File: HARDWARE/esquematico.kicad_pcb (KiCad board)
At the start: 2 copper layers, 52 parts, among them J1 Screw_Terminal_01x02, J10 LCD I2C, J12 Screw_Terminal_01x02, J13 Screw_Terminal_01x02, J14 Screw_Terminal_01x02, J15 Screw_Terminal_01x02, J2 Screw_Terminal_01x02, J3 Screw_Terminal_01x02, J4 Screw_Terminal_01x02, J5 Screw_Terminal_01x02, J6 PINERA, Q1 2N7000, Q2 2N7000, Q3 2N7000, Q4 2N7000, U1 PC817, U2 ESP32-DEVKITC-32D, U3 L7805, U4 PC817, U5 PC817, U6 PC817

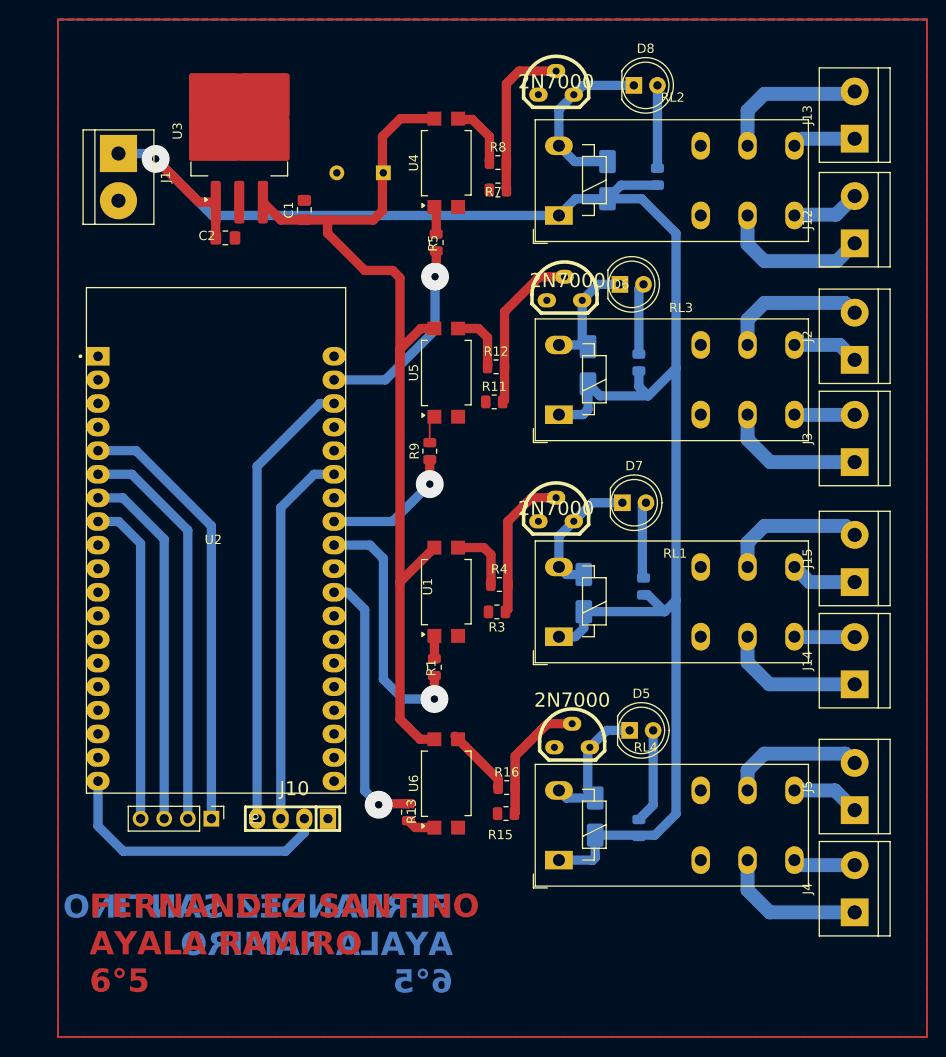
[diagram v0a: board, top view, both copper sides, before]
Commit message: terminamos la placa
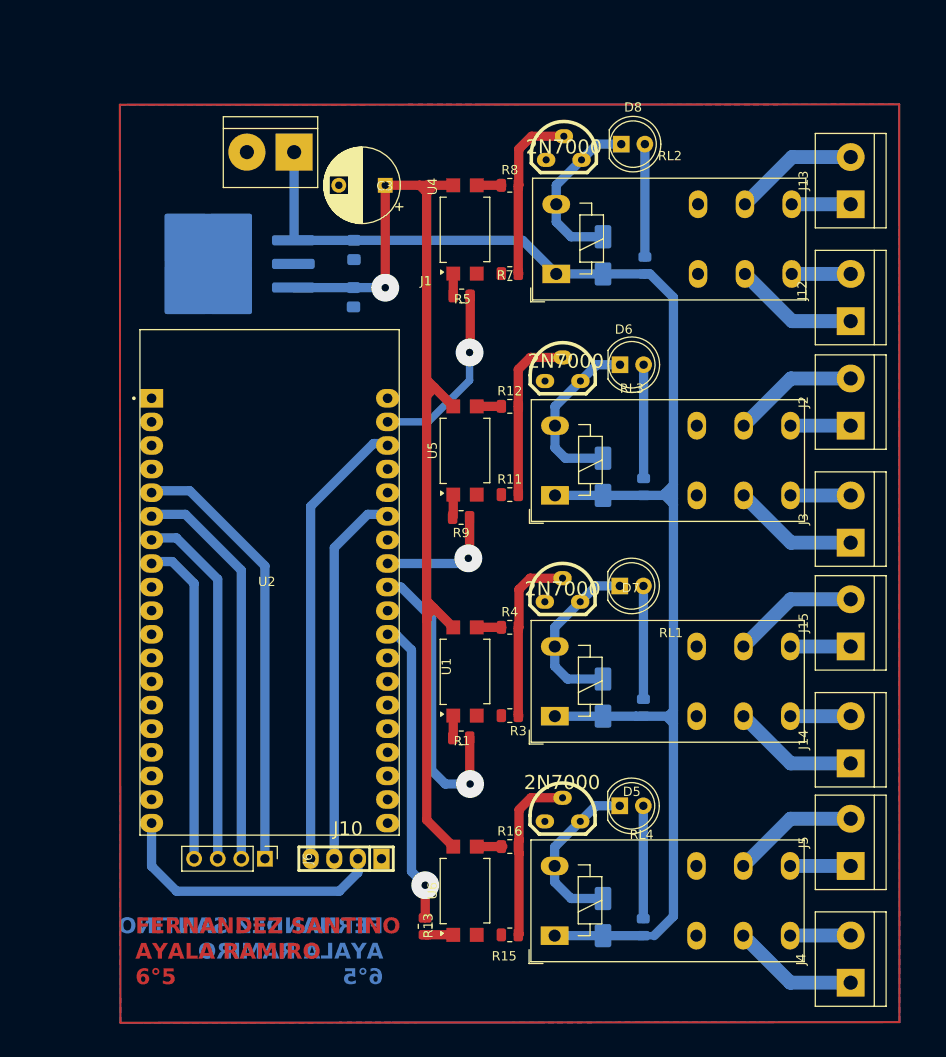
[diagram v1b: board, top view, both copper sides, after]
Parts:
- C1, C2, U3: moved to B.Cu
- C3: moved to F.Cu
- moved J1 18.9 mm to (91.9, 89.3), turned to 180 degrees
- moved U3 14.4 mm to (84.2, 101.3), turned to 180 degrees
- moved C2 13.9 mm to (98.3, 99.8), turned to -90 degrees
- moved R14 13.4 mm to (129.5, 125.3)
- moved R6 13.1 mm to (129.5, 149.1)
- moved R15 13.1 mm to (115.1, 173.5)
- moved R13 12.4 mm to (106.0, 172.6)
- moved D3 12.1 mm to (125.1, 124.2)
- moved U6 11.7 mm to (110.3, 168.8)
- moved D2 11.4 mm to (125.1, 148.0)
- moved R3 11.2 mm to (115.1, 149.9)
- moved D4 10.8 mm to (125.1, 171.6)
- moved C1 10.8 mm to (98.3, 104.9), turned to -90 degrees
- moved R2 10.7 mm to (129.5, 172.7)
- moved R11 10.1 mm to (115.1, 126.1)
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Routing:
- net 12V: track 201.1 -> 165.2 mm, vias 1 -> 0
- net +5V: track 103.4 -> 114.0 mm, vias 0 -> 1
- net Net-(D3-A): track 13.2 -> 18.9 mm
- net Net-(Q4-G): track 13.8 -> 18.7 mm
- net Net-(R16-Pad1): track 7.53 -> 2.80 mm
- net Net-(D6-A): track 7.71 -> 12.2 mm
- net GPIO18: track 27.8 -> 32.3 mm
- net Net-(R4-Pad1): track 7.17 -> 2.71 mm
- net Net-(D2-A): track 14.6 -> 18.8 mm
- net Net-(R12-Pad1): track 6.73 -> 2.64 mm
- net Net-(R8-Pad1): track 6.71 -> 2.70 mm
- net GPIO17: track 29.8 -> 33.6 mm
- net Net-(D7-A): track 8.54 -> 12.2 mm
- net Net-(D4-A): track 15.1 -> 18.5 mm
- net Net-(D8-A): track 8.91 -> 12.1 mm
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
